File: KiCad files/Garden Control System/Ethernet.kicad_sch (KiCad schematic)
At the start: 18 parts, among them J1 RJ45_Abracon_ARJP11A-MASA-B-A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, U2 DP83848C, Y1 25MHz

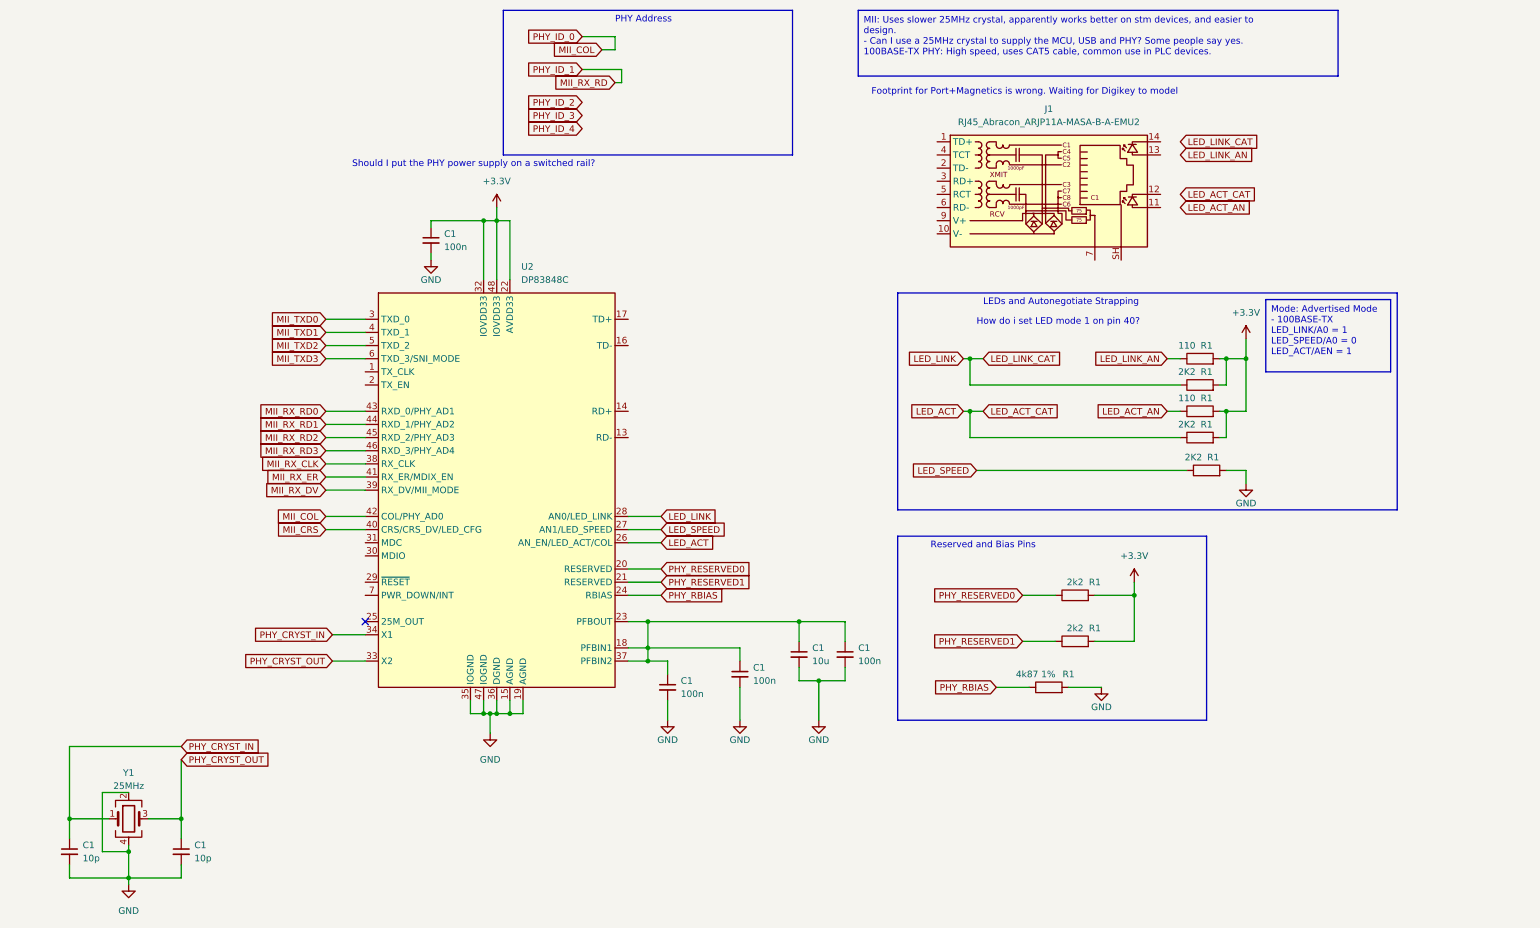
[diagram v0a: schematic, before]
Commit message: Close to finishing ethernet side
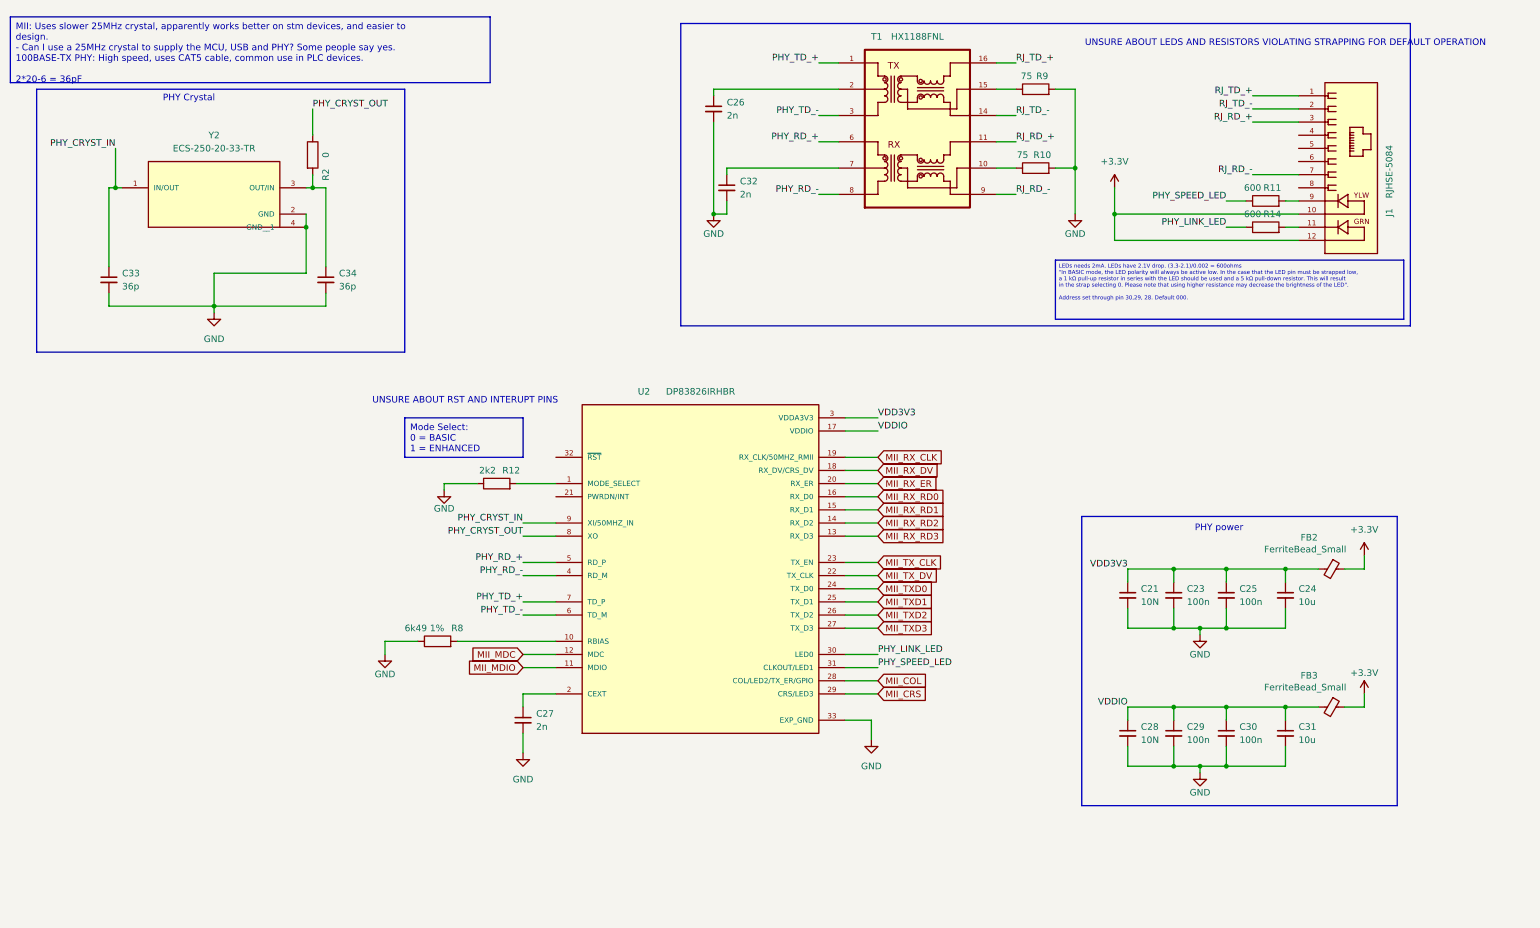
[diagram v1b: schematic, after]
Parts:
- removed C1: 100n, symbol Device:C_Small
- removed C1 (x2): 10p, symbol Device:C_Small
- removed J1: RJ45_Abracon_ARJP11A-MASA-B-A-EMU2, Connector_RJ:RJ45_Abracon_ARJP11A-MA_Horizontal, symbol Connector:RJ45_Abracon_ARJP11A-MASA-B-A-EMU2
- removed R1 (x3): 2K2, symbol Device:R
- removed R1: 4k87 1%, symbol Device:R
- removed R1 (x2): 110, symbol Device:R
- removed R1 (x2): 2k2, symbol Device:R
- removed U2: DP83848C, Package_QFP:LQFP-48_7x7mm_P0.5mm, symbol Interface_Ethernet:DP83848C
- removed Y1: 25MHz, symbol Device:Crystal_GND24
- added C26, C27, C32: 2n, symbol Device:C_Small
- added C28: 10N, symbol Device:C_Small
- added C29, C30: 100n, symbol Device:C_Small
- added C31: 10u, symbol Device:C_Small
- added C33, C34: 36p, symbol Device:C_Small
- added FB2, FB3: FerriteBead_Small, symbol Device:FerriteBead_Small
- added J1: RJHSE-5084, RJHSE-5084:AMPHENOL_RJHSE-5084, symbol RJHSE-5084:RJHSE-5084
- added R10, R9: 75, symbol Device:R
- added R11, R14: 600, symbol Device:R
- added R12: 2k2, symbol Device:R
- added R2: 0, symbol Device:R
- added R8: 6k49 1%, symbol Device:R
- added T1: HX1188FNL, HX1188FNL:HXXXX, symbol HX1188FNL:HX1188FNL
- added U2: DP83826IRHBR, DP83826IRHBR:IC_DP83826IRHBR, symbol DP83826IRHBR:DP83826IRHBR
- added Y2: ECS-250-20-33-TR, ECS-250-20-33-TR:XTAL_ECS-250-20-33-TR, symbol ECS-250-20-33-TR:ECS-250-20-33-TR
- C21: renamed from C1; value 100n -> 10N
- renumbered C1 to C23, C1 to C24, C1 to C25
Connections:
- net +3.3V: now also FB2.1, FB3.1, J1.10, J1.12
- net GND: now also C26.2, C27.2, C28.2, C29.2, C30.2, C31.2, C32.2, C33.2, C34.2, R10.2, R12.1, R8.1, R9.2, U2.33 (EXP_GND), Y2.2 (GND), Y2.4 (GND__1)
- net MII_COL: now also U2.28 (COL/LED2/TX_ER/GPIO)
- net MII_CRS: now also U2.29 (CRS/LED3)
- net MII_RX_CLK: now also U2.19 (RX_CLK/50MHZ_RMII)
- net MII_RX_DV: now also U2.18 (RX_DV/CRS_DV)
- net MII_RX_ER: now also U2.20 (RX_ER)
- net MII_RX_RD0: now also U2.16 (RX_D0)
- net MII_RX_RD1: now also U2.15 (RX_D1)
- net MII_RX_RD2: now also U2.14 (RX_D2)
- net MII_RX_RD3: now also U2.13 (RX_D3)
- net MII_TXD0: now also U2.24 (TX_D0)
- net MII_TXD1: now also U2.25 (TX_D1)
- net MII_TXD2: now also U2.26 (TX_D2)
- net MII_TXD3: now also U2.27 (TX_D3)
- net PHY_CRYST_IN: now also C33.1, U2.9 (XI/50MHZ_IN), Y2.1 (IN/OUT)
- net PHY_CRYST_OUT: now also R2.1, U2.8 (XO)
- net VDD3V3: now reaches C21.1, C23.1, C24.1, C25.1
- net VDD3V3: now also FB2.2, U2.3 (VDDA3V3)
- new net: C34.1, R2.2, Y2.3 (OUT/IN)
- new net: R9.1, T1.15
- new net: C27.1, U2.2 (CEXT)
- new net: J1.9, R11.2
- new net: R10.1, T1.10
- new net: R12.2, U2.1 (MODE_SELECT)
- new net: R8.2, U2.10 (RBIAS)
- new net: C32.1, T1.7
- new net: C26.1, T1.2
- new net: J1.11, R14.2
- new net MII_MDC: U2.12 (MDC)
- new net MII_MDIO: U2.11 (MDIO)
- new net MII_TX_CLK: U2.23 (TX_EN)
- new net MII_TX_DV: U2.22 (TX_CLK)
- new net PHY_LINK_LED: R14.1, U2.30 (LED0)
- new net PHY_RD_+: T1.6, U2.5 (RD_P)
- new net PHY_RD_-: T1.8, U2.4 (RD_M)
- new net PHY_SPEED_LED: R11.1, U2.31 (CLKOUT/LED1)
- new net PHY_TD_+: T1.1, U2.7 (TD_P)
- new net PHY_TD_-: T1.3, U2.6 (TD_M)
- new net RJ_RD_+: J1.3, T1.11
- new net RJ_RD_-: J1.7, T1.9
- new net RJ_TD_+: J1.1, T1.16
- new net RJ_TD_-: J1.2, T1.14
- new net VDDIO: C28.1, C29.1, C30.1, C31.1, FB3.2, U2.17 (VDDIO)
- no-connect marks 1 -> 0
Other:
- note added: "PHY Crystal"
- note added: "PHY power"
- note added: "UNSURE ABOUT LEDS AND RESISTORS VIOLATING STRAPPING FOR DEFAULT OPERATION"
- note added: "UNSURE ABOUT RST AND INTERUPT PINS"
- note removed: "Footprint for Port+Magnetics is wrong. Waiting for Digikey to model"
- note removed: "How do i set LED mode 1 on pin 40?"
- note removed: "LEDs and Autonegotiate Strapping"
- note removed: "PHY Address"
- note removed: "Reserved and Bias Pins"
- note removed: "Should I put the PHY power supply on a switched rail?"
- moved on the sheet: C21, C23, C24, C25
